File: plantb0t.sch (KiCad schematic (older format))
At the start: 32 parts

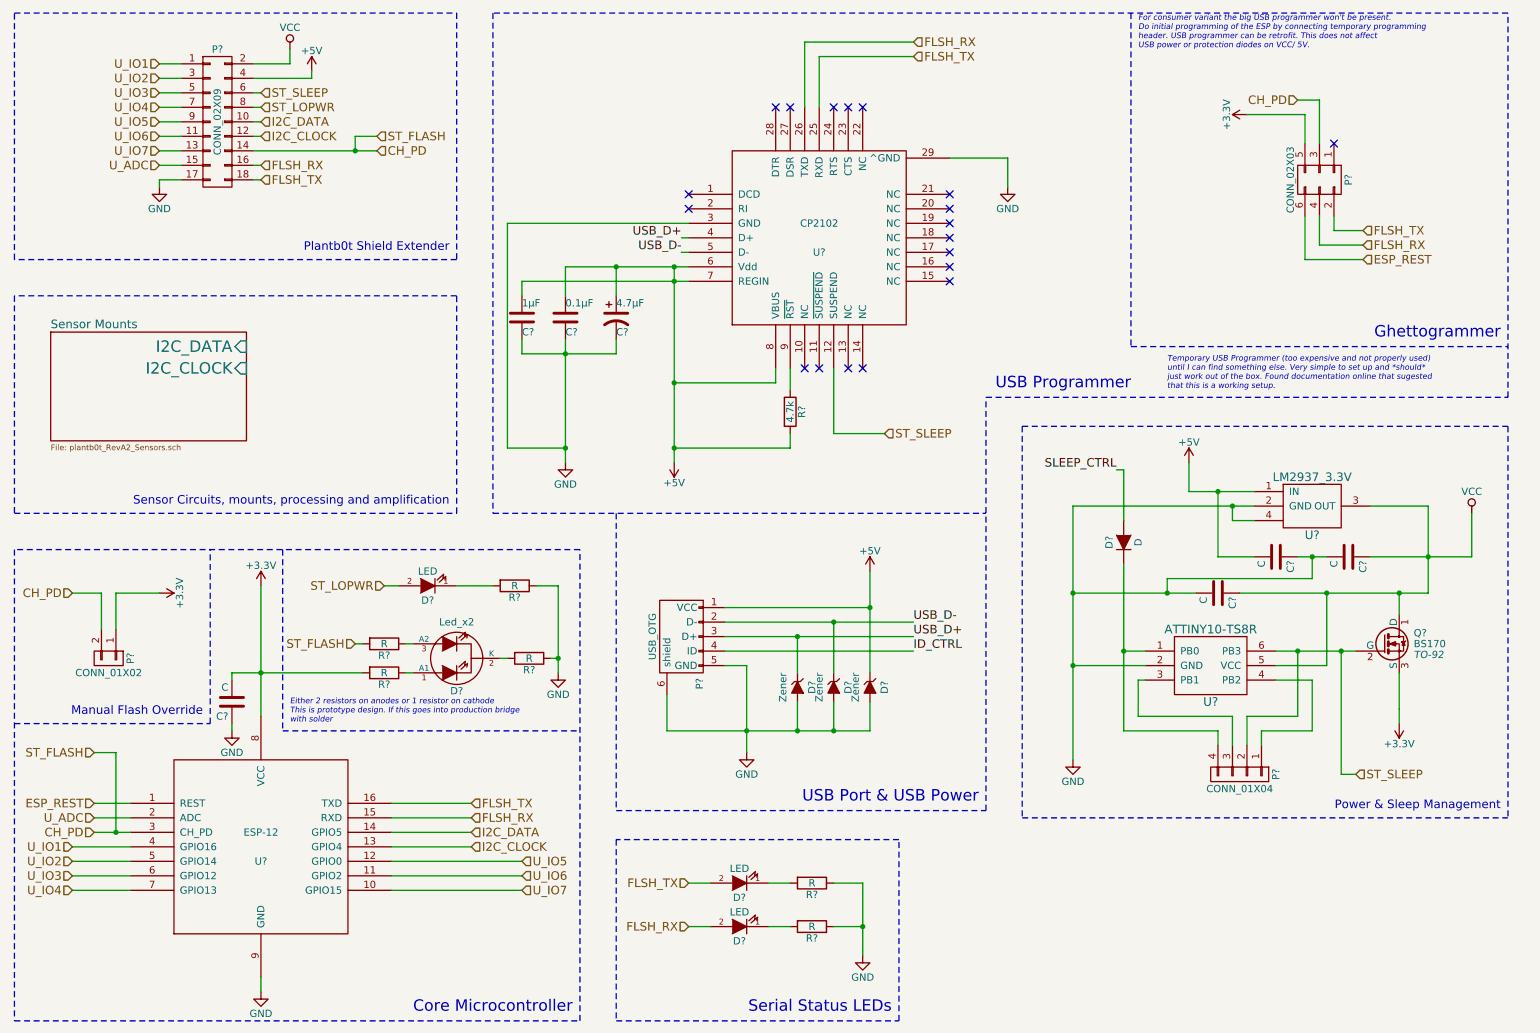
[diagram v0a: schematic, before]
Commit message: Updating a lot of stuff...
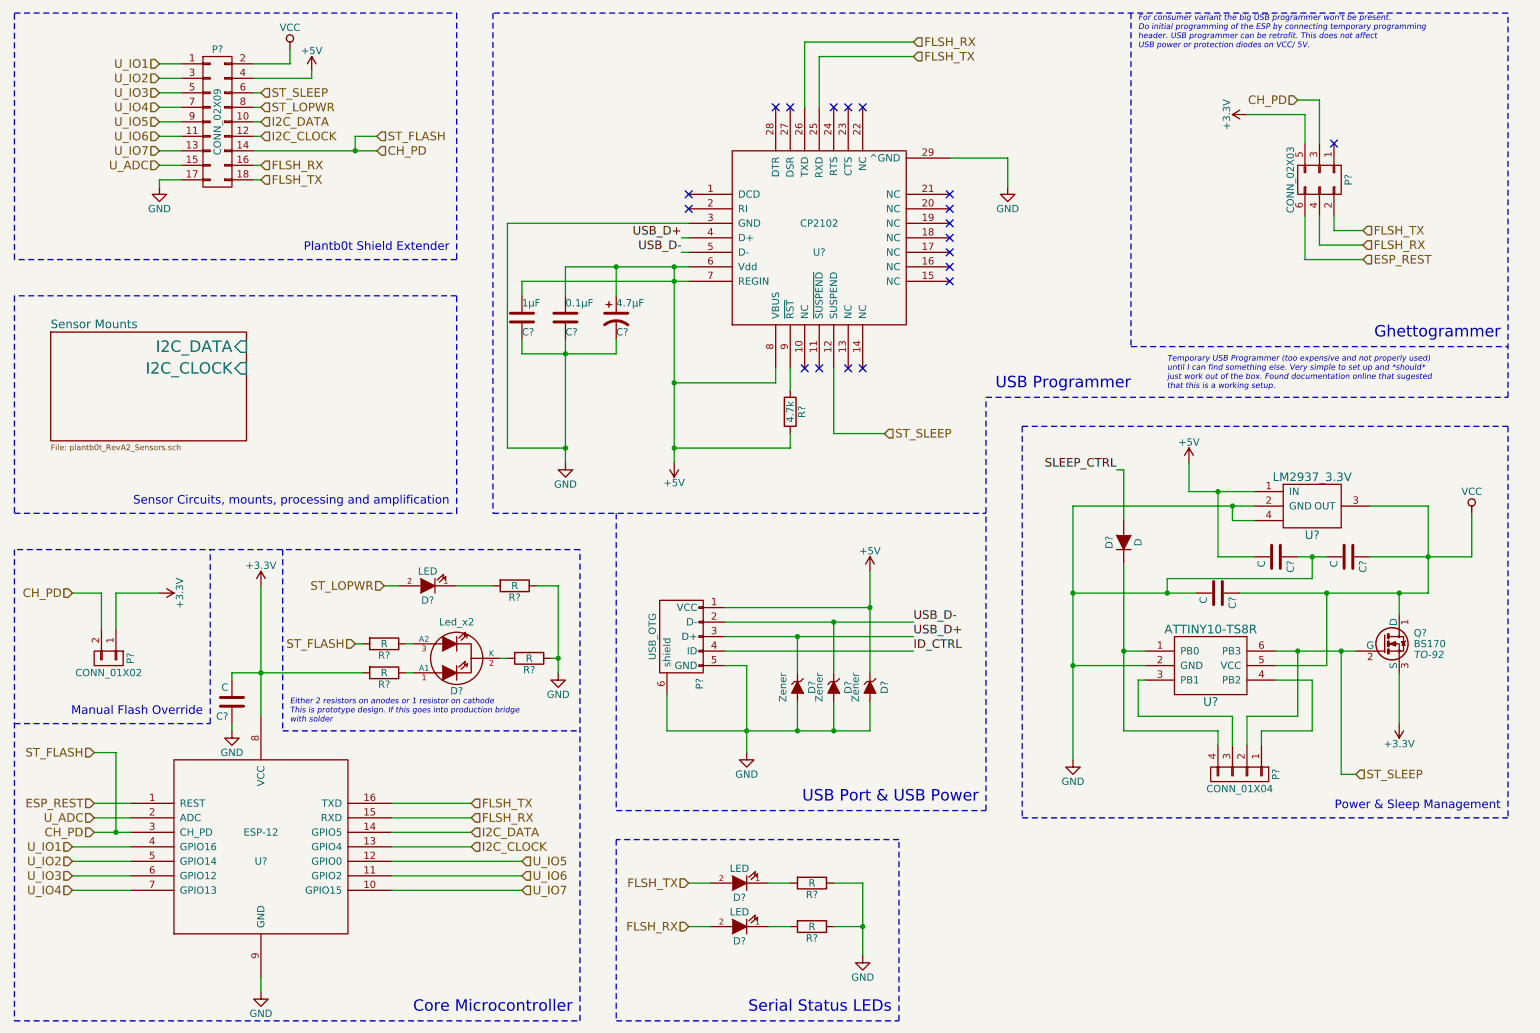
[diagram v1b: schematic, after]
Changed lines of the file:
@@
 LIBS:valves
 LIBS:kookie_power
-LIBS:kookie_logic
 LIBS:kookie_mcu
+LIBS:kookie_sensors
 LIBS:ESP8266
-LIBS:kookie_sensors
 LIBS:plantb0t-cache
 EELAYER 25 0
@@
 	2350 7350 2350 7450
 Wire Wire Line
-	2350 4650 2350 5250
-Wire Wire Line
-	2350 5250 2350 5550
+	2350 4650 2350 5550
 Wire Wire Line
 	3050 5050 3000 5050
 Wire Wire Line
-	4400 4650 4400 5150
-Wire Wire Line
-	4400 5150 4400 5250
+	4400 4650 4400 5250
 Wire Wire Line
 	3250 6150 3800 6150
@@
 	650  2650 650  4150
 Wire Wire Line
-	9350 5100 9500 5100
-Wire Wire Line
-	9500 5100 9800 5100
-Wire Wire Line
-	9800 5100 9900 5100
+	9350 5100 9900 5100
 Wire Wire Line
 	9700 5200 9350 5200
 Wire Wire Line
-	10200 5250 10200 5500
-Wire Wire Line
-	10200 5500 10200 5600
-Wire Wire Line
-	7950 4100 7950 4700
-Wire Wire Line
-	7950 4700 7950 5200
-Wire Wire Line
-	7950 5200 7950 5850
+	10200 5250 10200 5600
+Wire Wire Line
+	7950 4100 7950 5850
 Wire Wire Line
 	7950 5200 8450 5200
@@
 Connection ~ 7950 4700
 Wire Wire Line
-	9500 4450 9600 4450
-Wire Wire Line
-	9600 4450 9700 4450
-Wire Wire Line
-	8750 4000 8950 4000
-Wire Wire Line
-	8950 4000 9200 4000
+	9500 4450 9700 4450
+Wire Wire Line
+	8750 4000 9200 4000
 Wire Wire Line
 	8950 4000 8950 4450
@@
 	8950 4450 9200 4450
 Wire Wire Line
-	7950 4100 9050 4100
-Wire Wire Line
-	9050 4100 9200 4100
+	7950 4100 9200 4100
 Wire Wire Line
 	9050 4100 9050 4200
@@
 Connection ~ 8950 4000
 Wire Wire Line
-	10400 4700 10400 4450
-Wire Wire Line
-	10400 4450 10400 4100
-Wire Wire Line
-	10000 4450 10400 4450
-Wire Wire Line
-	10400 4450 10700 4450
+	10400 4700 10400 4100
+Wire Wire Line
+	10000 4450 10700 4450
 Wire Notes Line
 	7600 3550 10950 3550
@@
 	8300 3850 8300 4200
 Wire Wire Line
-	8300 4500 8300 5100
-Wire Wire Line
-	8300 5100 8300 5650
-Wire Wire Line
-	2150 5250 2350 5250
-Wire Wire Line
-	2350 5250 3050 5250
+	8300 4500 8300 5650
+Wire Wire Line
+	2150 5250 3050 5250
 Connection ~ 2350 5250
 Wire Wire Line
 	1200 6250 1450 6250
 Wire Wire Line
-	1200 6350 1350 6350
-Wire Wire Line
-	1350 6350 1450 6350
+	1200 6350 1450 6350
 Wire Wire Line
 	1650 1750 1800 1750
 Wire Wire Line
-	2300 1650 3000 1650
-Wire Wire Line
-	3000 1650 3150 1650
+	2300 1650 3150 1650
 Wire Wire Line
 	3200 4650 3300 4650
@@
 	5150 5400 5150 5650
 Wire Wire Line
-	5150 5650 5700 5650
-Wire Wire Line
-	5700 5650 6050 5650
-Wire Wire Line
-	6050 5650 6300 5650
-Wire Wire Line
-	6300 5650 6550 5650
+	5150 5650 6550 5650
 Wire Wire Line
 	5550 5200 5700 5200
 Wire Wire Line
-	5700 5200 5700 5650
-Wire Wire Line
-	5700 5650 5700 5800
+	5700 5200 5700 5800
 Connection ~ 5700 5650
 Wire Wire Line
@@
 Connection ~ 6300 5650
 Wire Wire Line
-	5550 5000 6050 5000
-Wire Wire Line
-	6050 5000 6850 5000
-Wire Wire Line
-	5550 4900 6300 4900
-Wire Wire Line
-	6300 4900 6850 4900
+	5550 5000 6850 5000
+Wire Wire Line
+	5550 4900 6850 4900
 Wire Wire Line
 	6050 5250 6050 5000
@@
 	5550 4800 6550 4800
 Wire Wire Line
-	6550 4550 6550 4800
-Wire Wire Line
-	6550 4800 6550 5250
+	6550 4550 6550 5250
 Connection ~ 6550 4800
 Wire Wire Line
@@
 	9800 5950 9900 5950
 Wire Wire Line
-	9100 4700 9700 4700
-Wire Wire Line
-	9700 4700 10200 4700
-Wire Wire Line
-	10200 4700 10400 4700
+	9100 4700 10400 4700
 Wire Wire Line
 	10200 4700 10200 4850
@@
 Connection ~ 8600 4700
 Wire Wire Line
-	7950 4700 8600 4700
-Wire Wire Line
-	8600 4700 8800 4700
+	7950 4700 8800 4700
 Wire Wire Line
 	8600 4700 8600 4600
@@
 	6300 7000 6500 7000
 Wire Wire Line
-	6500 6700 6500 7000
-Wire Wire Line
-	6500 7000 6500 7200
+	6500 6700 6500 7200
 Wire Wire Line
 	6500 6700 6300 6700
@@
 	6000 3150 6000 3150
 Wire Wire Line
-	4150 3050 4450 3050
-Wire Wire Line
-	4450 3050 4800 3050
-Wire Wire Line
-	4450 2950 4450 3050
-Wire Wire Line
-	4450 3050 4450 3700
-Wire Wire Line
-	4450 3700 4450 3800
+	4150 3050 4800 3050
+Wire Wire Line
+	4450 2950 4450 3800
 Wire Wire Line
 	4800 3050 4800 2950
@@
 Connection ~ 4450 3700
 Wire Wire Line
-	4150 2550 5200 2550
-Wire Wire Line
-	5200 2550 5300 2550
+	4150 2550 5300 2550
 Connection ~ 5200 2550
 Wire Wire Line
-	4450 2450 4800 2450
-Wire Wire Line
-	4800 2450 5200 2450
-Wire Wire Line
-	5200 2450 5300 2450
+	4450 2450 5300 2450
 Connection ~ 5200 2450
 Wire Wire Line
@@
 	6300 3600 6650 3600
 Wire Wire Line
-	5200 2450 5200 2550
-Wire Wire Line
-	5200 2550 5200 3250
-Wire Wire Line
-	5200 3250 5200 3700
-Wire Wire Line
-	5200 3700 5200 3800
+	5200 2450 5200 3800
 Wire Wire Line
 	5900 3250 5900 3150
